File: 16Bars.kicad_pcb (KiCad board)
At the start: 2 copper layers, 28.5 x 105 mm, 49 parts, among them IC1 CD4033BE, IC2 CD4033BE, IC3 CD4510BE, IC4 CD4510BE, IC5 CD4510BE, J1 3.5mm_Mono_Switched, J2 Conn_02x05_Odd_Even, Q1 2N3904, Q2 2N3904, Q3 2N3904, SW1 SW_Push_LED_Thonk_Low_Profile, SW2 SW_SPDT - EG1249, SW3 SW_SPDT-EG1249

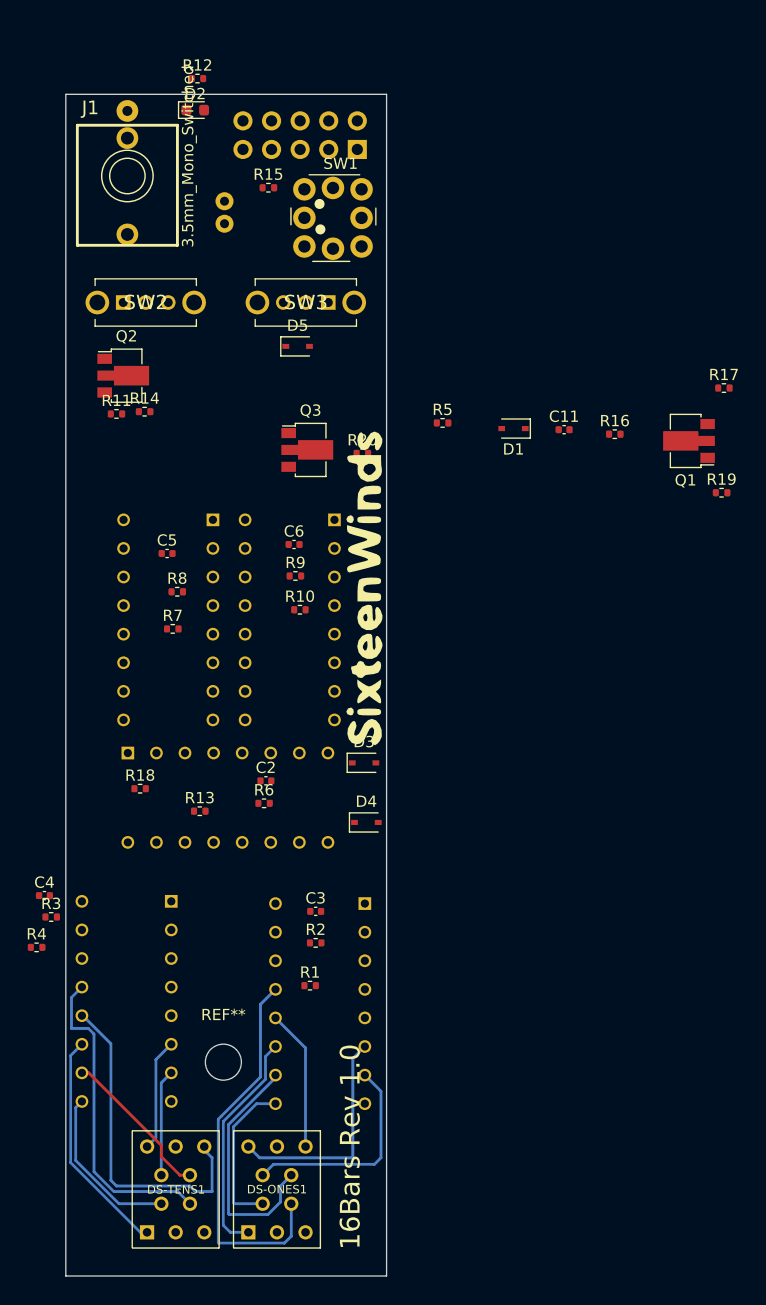
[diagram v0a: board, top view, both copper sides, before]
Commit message: More PCB Layout
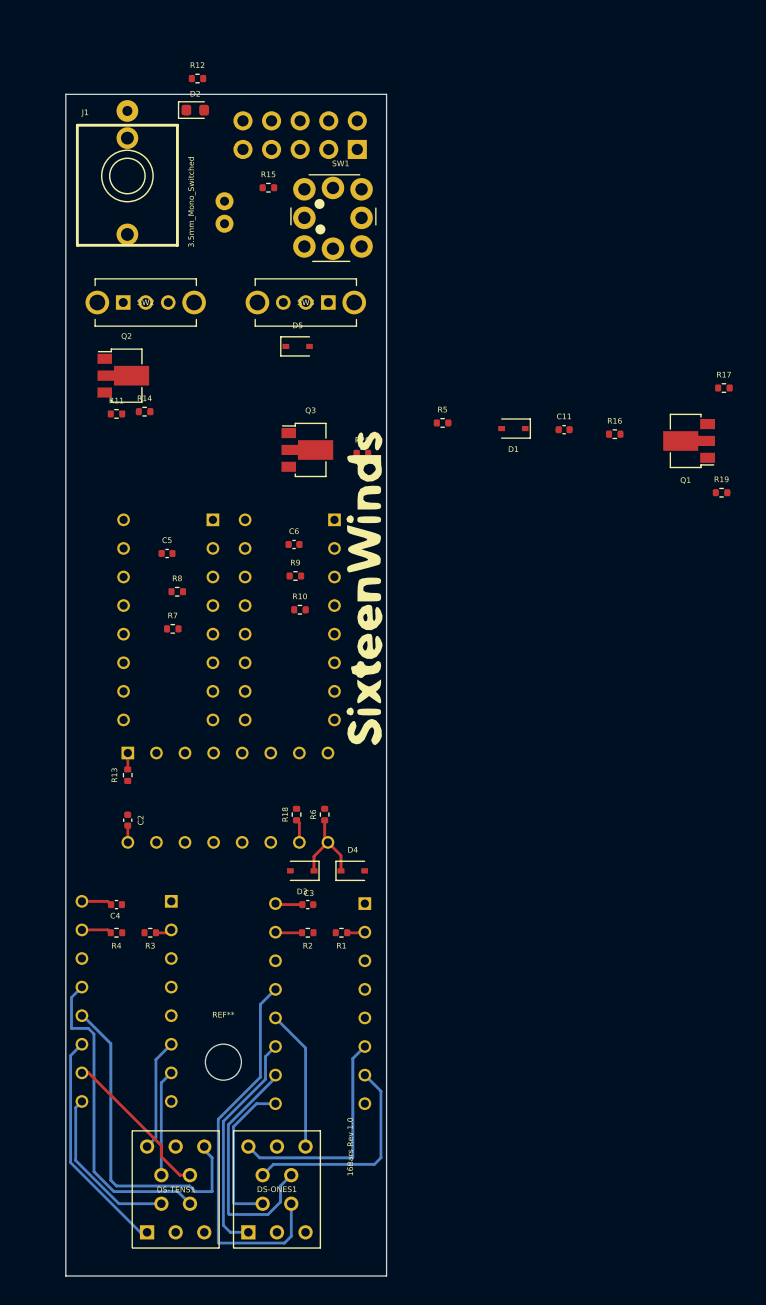
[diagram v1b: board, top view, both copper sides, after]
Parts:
- moved R18 14.1 mm to (77.0, 99.0), turned to -90 degrees
- moved C2 12.8 mm to (62.0, 99.5), turned to -90 degrees
- moved D3 11.1 mm to (77.5, 104.0), turned to 180 degrees
- moved R3 8.91 mm to (64.0, 109.5), turned to 180 degrees
- moved R4 7.22 mm to (61.0, 109.5), turned to 180 degrees
- moved R13 7.16 mm to (62.0, 95.5), turned to 90 degrees
- moved C4 6.45 mm to (61.0, 107.0), turned to 180 degrees
- moved R6 5.48 mm to (79.5, 99.0), turned to -90 degrees
- moved R1 5.47 mm to (81.0, 109.5), turned to 180 degrees
- moved D4 4.46 mm to (82.0, 104.0)
- moved R2 1.14 mm to (78.0, 109.5), turned to 180 degrees
- moved C3 0.92 mm to (78.0, 107.0), turned to 180 degrees
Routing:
- net Net-(D3-Pad1): track 0.00 -> 8.13 mm
- net +12V: track 0.00 -> 6.63 mm
- net /RESET: track 0.00 -> 5.04 mm
- net Net-(IC3-Pad10): track 0.00 -> 2.08 mm
- net Net-(IC1-Pad2): track 0.00 -> 1.59 mm
- net Net-(IC3-Pad1): track 0.00 -> 1.46 mm
- net Net-(IC2-Pad2): track 0.00 -> 1.46 mm
